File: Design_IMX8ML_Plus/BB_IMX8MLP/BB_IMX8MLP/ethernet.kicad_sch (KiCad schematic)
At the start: 3 parts, among them J5 RJ45_Amphenol_RJMG1BD3B8K1ANR, J6 RJ45_Amphenol_RJMG1BD3B8K1ANR, U1 KSZ9131RNXI

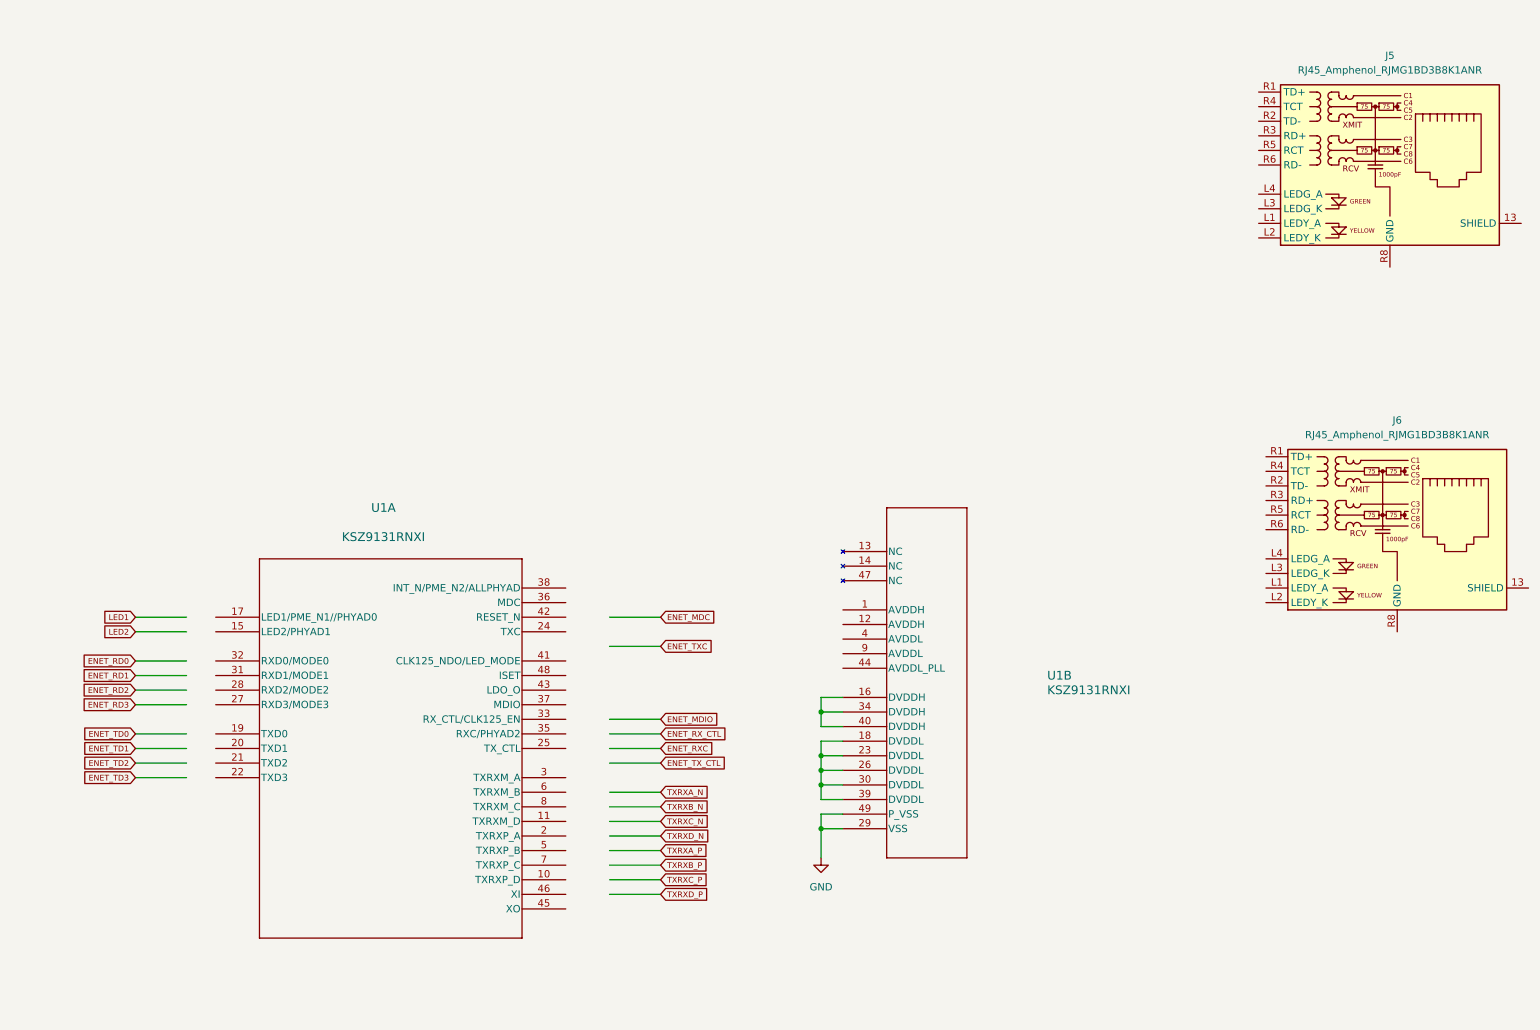
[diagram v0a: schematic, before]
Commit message: improving the usb conector
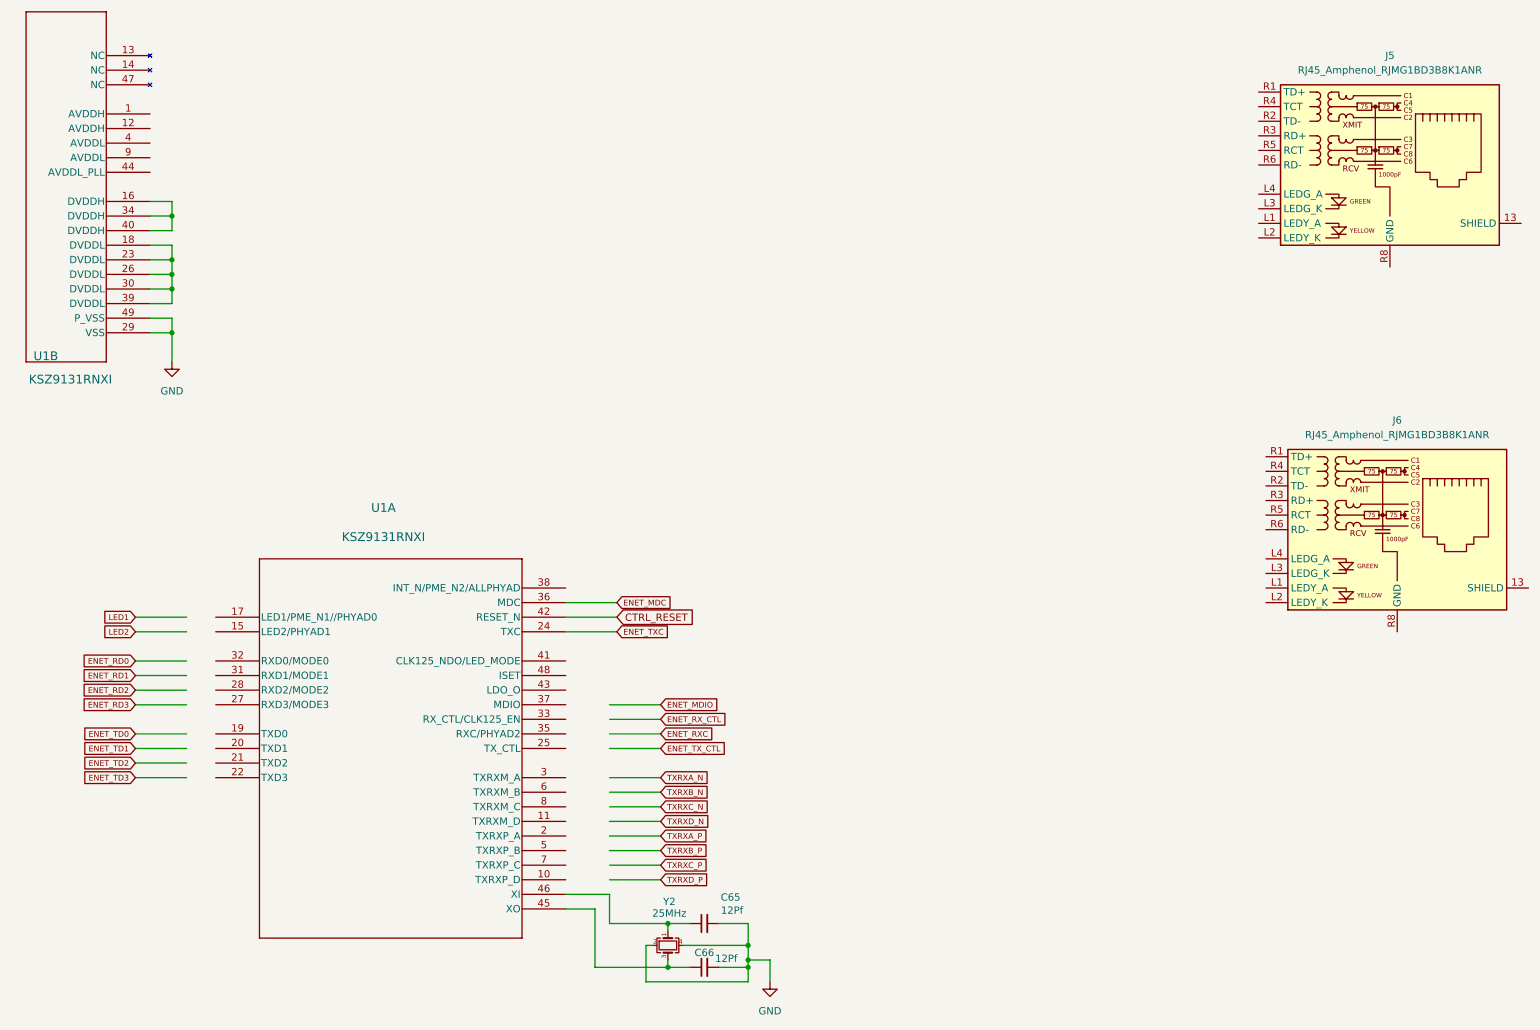
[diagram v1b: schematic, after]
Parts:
- added C65, C66: 12Pf, Capacitor_SMD:C_0402_1005Metric, symbol Device:C_Small
- added Y2: 25MHz, Crystal:Crystal_SMD_0603-4Pin_6.0x3.5mm, symbol Device:Crystal_GND24_Small
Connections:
- net ENET_MDC: now also U1.36 (MDC)
- net ENET_TXC: now also U1.24 (TXC)
- net GND: now also C65.2, C66.2, Y2.2, Y2.4
- net CTRL_RESET: now reaches U1.42 (RESET_N)
- net at U1.45 (XO): now also C66.1, Y2.3
- net at U1.46 (XI): now also C65.1, Y2.1
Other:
- moved on the sheet: U1B
